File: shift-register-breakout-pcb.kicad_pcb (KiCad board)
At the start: 2 copper layers, 74 x 44 mm, 28 parts, among them J1 Conn_01x08_Socket, J2 Conn_01x08_Socket, J3 Conn_01x08_Socket, J4 Conn_01x08_Socket, J5 Conn_01x08_Socket, J6 Conn_01x03_Socket

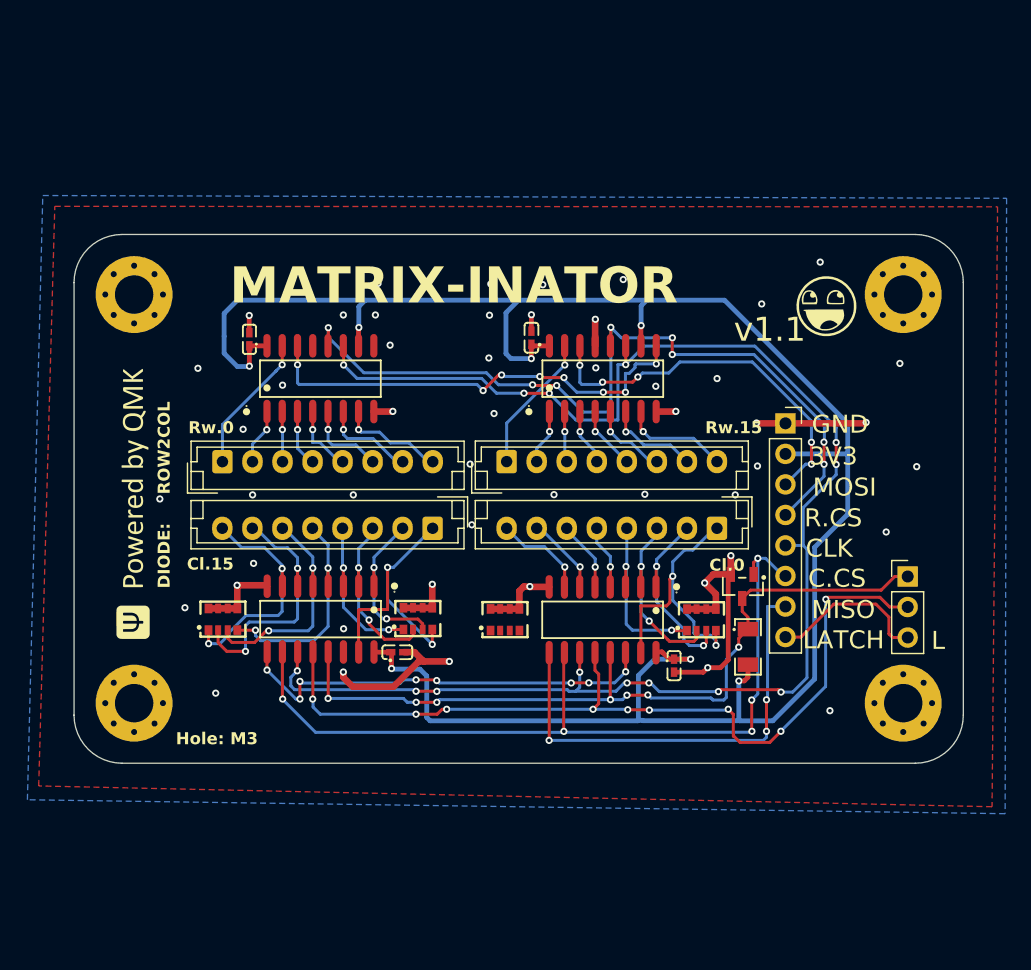
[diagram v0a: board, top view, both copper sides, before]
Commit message: vik-i-fying the design
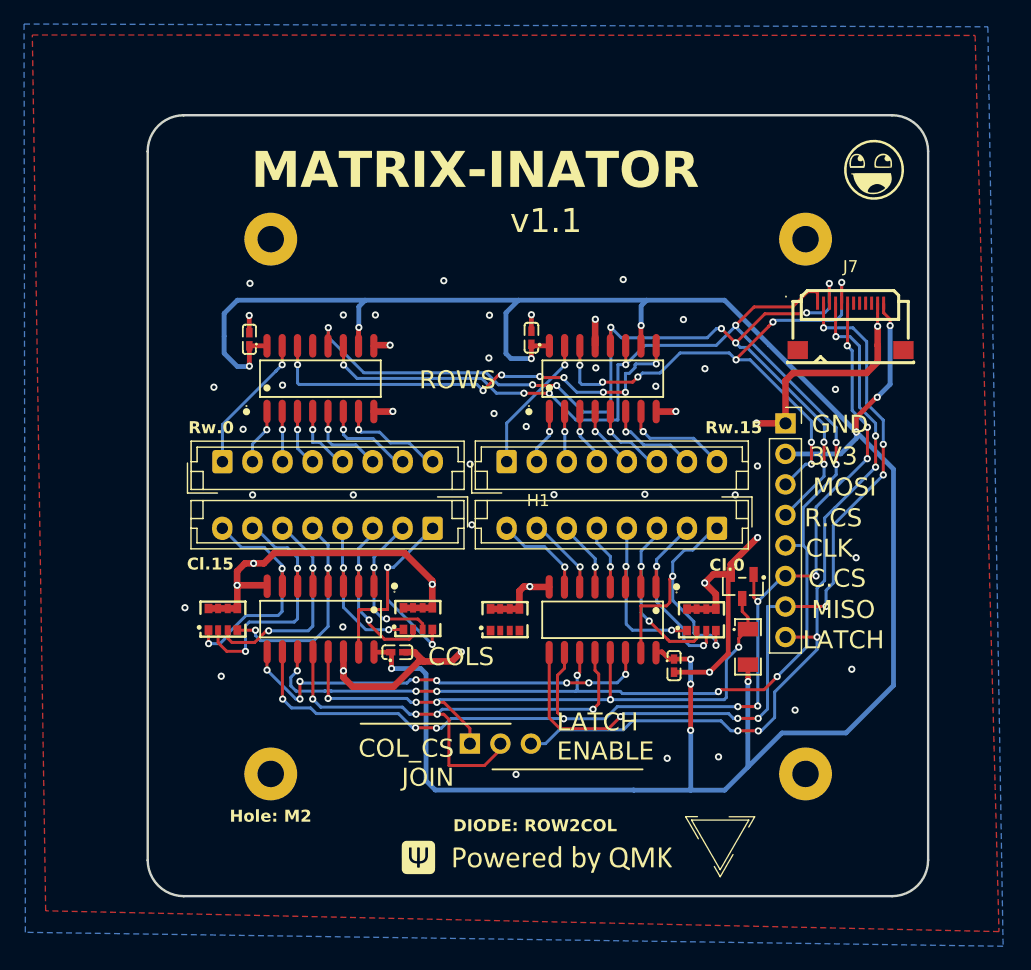
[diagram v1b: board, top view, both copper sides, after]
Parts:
- removed H2, H3, H4: MountingHole, MountingHole:MountingHole_3.2mm_M3_Pad_Via
- added FID1: Fiducial, vik:vik-logo-small, F.Cu at (121.8, 98.2)
- added J7: vik-module-connector, ct-kicad:FPC-SMD_XF2M-1215-1AH, F.Cu at (132.6, 55.7)
- H1: footprint MountingHole:MountingHole_3.2mm_M3_Pad_Via -> vik:vik-module-mounting-large
- J6: moved to B.Cu
- moved LOGO2 44.5 mm to (106.4, 99.8), turned to 0 degrees
- moved J6 39.0 mm to (100.9, 90.4), turned to -90 degrees
- moved H1 38.0 mm to (106.6, 70.6)
- moved LOGO1 12.0 mm to (134.6, 42.6)
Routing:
- net COL_LATCH: track 13.4 -> 64.5 mm, vias 0 -> 6
- net GND: track 68.9 -> 104.7 mm
- net +3V3: track 171.3 -> 206.1 mm, vias 7 -> 12
- net SPI_MISO: track 37.9 -> 69.1 mm, vias 3 -> 7
- net Net-(J6-Pin_2): track 71.4 -> 43.3 mm, vias 9 -> 4
- net COL_CS: track 69.8 -> 93.3 mm, vias 5 -> 11
- net SPI_MOSI: track 31.6 -> 47.1 mm, vias 5 -> 8
- net ROW_CS: track 67.8 -> 80.3 mm, vias 8 -> 10
- net COL_CS_MOS: track 65.3 -> 55.3 mm, vias 7 -> 5
- net SPI_CLK: track 128.7 -> 138.5 mm, vias 14 -> 13
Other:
- board size 74 x 44 mm -> 64.9 x 65 mm
- board text added: "COLS"
- board text added: "COL_CS JOIN"
- board text added: "Hole: M2"
- board text added: "LATCH ENABLE"
- board text added: "ROWS"
- board text removed: "Hole: M3"
- board text removed: "L"
